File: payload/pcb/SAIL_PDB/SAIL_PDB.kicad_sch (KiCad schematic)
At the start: 45 parts, among them J1 440055-6_6POS_2MM, P1 OSTTE020104, P2 OSTTE020104, P3 OSTTE020104, P4 OSTTE020104, P5 OSTTE020104, P6 OSTTE020104, U1 AP63357_(SparkFun_Buck_Regula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, U2 DMN3051L-7, U3 AP63203, U4 DMN3051L-7

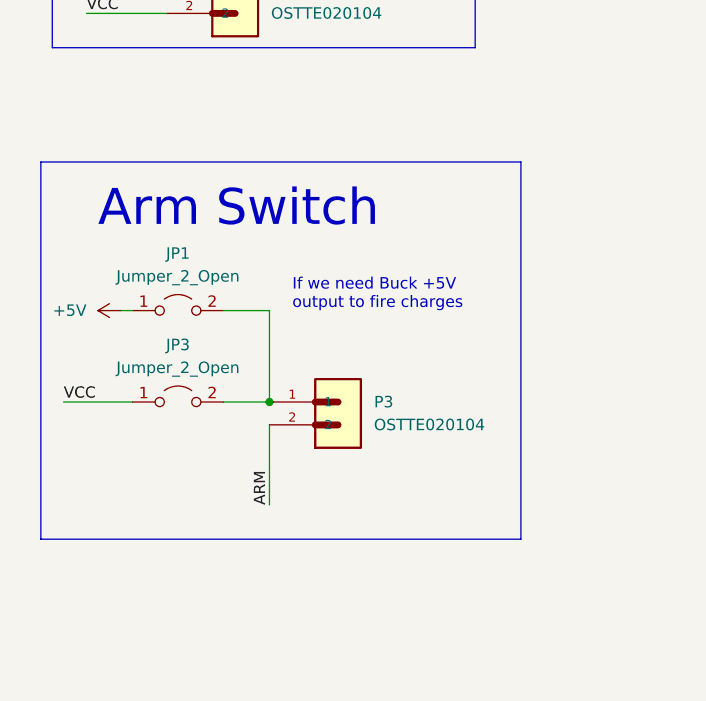
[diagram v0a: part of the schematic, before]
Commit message: Updated PCBs
im dumb
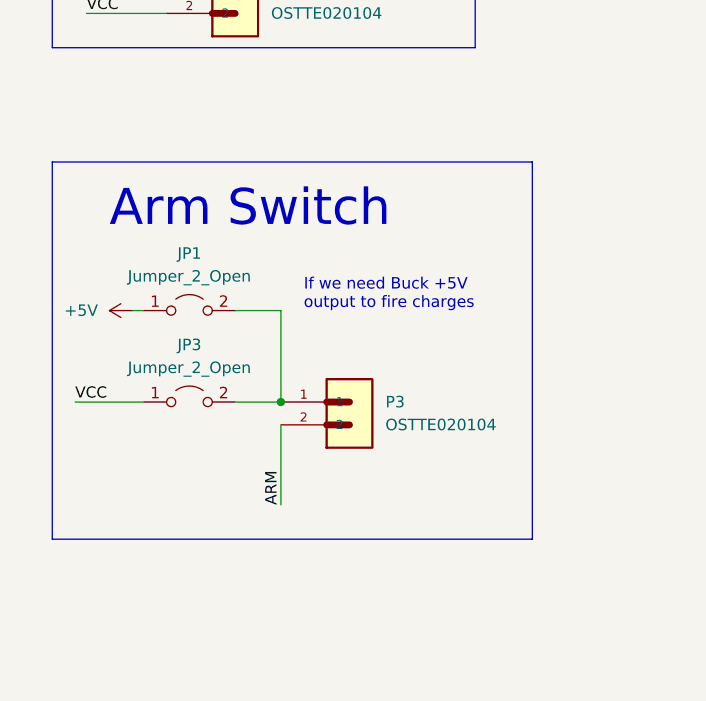
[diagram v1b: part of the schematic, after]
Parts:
- C1, C6: Distributor Part Number (none) -> 445-14418-1-ND
- C10: Distributor Part Number (none) -> 1276-1029-1-ND
- C2, C7: Distributor Part Number (none) -> 311-1140-1-ND
- C3: Distributor Part Number (none) -> 478-KGM21BCG1H4R7BTCT-ND
- C4, C5, C8, C9: Distributor Part Number (none) -> 445-14428-1-ND
- H1, H2, H3, H4: Distributor Part Number (none) -> -; Price (none) -> -; Type (none) -> -
- J1: Distributor Part Number (none) -> A100047-ND
- JP1, JP3: Distributor (none) -> -; Distributor Part Number (none) -> -; Item # (none) -> 10; MANUFACTURER (none) -> -; Mfg Part # (none) -> -; Notes (none) -> -; Package/Footprint (none) -> -; Price (none) -> -; Produce Page (none) -> -; Type (none) -> -
- L1: Distributor Part Number (none) -> 445-173057-1-ND; Item # 10 -> 11
- L2: Distributor Part Number (none) -> 587-2893-1-ND; Item # 11 -> 12
- P1, P2, P3, P4, P5, P6: Distributor Part Number (none) -> ED2740-ND; Item # 12 -> 13
- R1: Distributor Part Number (none) -> RMCF0805FT3K90CT-ND; Item # 20 -> 21
- R10: Distributor Part Number (none) -> PPC3.9W-1CT-ND; Item # 15 -> 20; MANUFACTURER Stackpole Electronics Inc -> (none); Mfg Part # RMCF0805FT470R -> (none); Produce Page https://www.digikey.com/en/products/detail/stackpole-electr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 -> https://www.digikey.com/en/products/detail/vishay-beyschlag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; Type SMD -> THT
- R2: Distributor Part Number (none) -> RMCF0805FT3K60CT-ND; Item # 14 -> 15
- R2, R3, R9: Distributor Part Number (none) -> RMCF0805FT470RCT-ND; Item # 15 -> 16
- R2: Distributor Part Number (none) -> 2019-RK73B2ATTD683JCT-ND; Item # 13 -> 14
- R2: Distributor Part Number (none) -> RMCF0805FT30K0CT-ND; Item # 17 -> 18
- R2: Distributor Part Number (none) -> 311-158KCRCT-ND; Item # 16 -> 17
- R6: Distributor Part Number (none) -> S2.7HCT-ND; Item # 18 -> 15; MANUFACTURER Stackpole Electronics Inc -> (none); Mfg Part # RMCF0805FT5R60 -> (none); Produce Page https://www.digikey.com/en/products/detail/stackpole-electronics-inc/RMCF0805FT5R60/1713196 -> https://www.digikey.com/en/products/detail/stackpole-electronics-inc/CFM12JT2R70/1741892; Type SMD -> THT
- TP1, TP2, TP3, TP4: Distributor (none) -> DigiKey; Distributor Part Number (none) -> 36-5015CT-ND; Item # (none) -> 22; MANUFACTURER (none) -> Keystone Electronics; Mfg Part # (none) -> 5015; Price (none) -> $0.45; Produce Page (none) -> https://www.digikey.com/en/products/detail/keystone-electro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; Type (none) -> SMD
- U1: Distributor Part Number (none) -> 31-AP63357DV-7CT-ND; Item # 22 -> 23
- U2, U4: Distributor Part Number (none) -> DMN3051LDICT-ND
- U3: Distributor Part Number (none) -> AP63203WU-7DICT-ND; Item # 23 -> 25
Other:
- moved on the sheet: JP1, JP3, P3
